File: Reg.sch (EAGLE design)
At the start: 25 parts, among them Q1 NPN, Q2 NPN, Q3 PNP, Q4 NPN, Q5 NPN, Q6 NPN, Q8 PNP

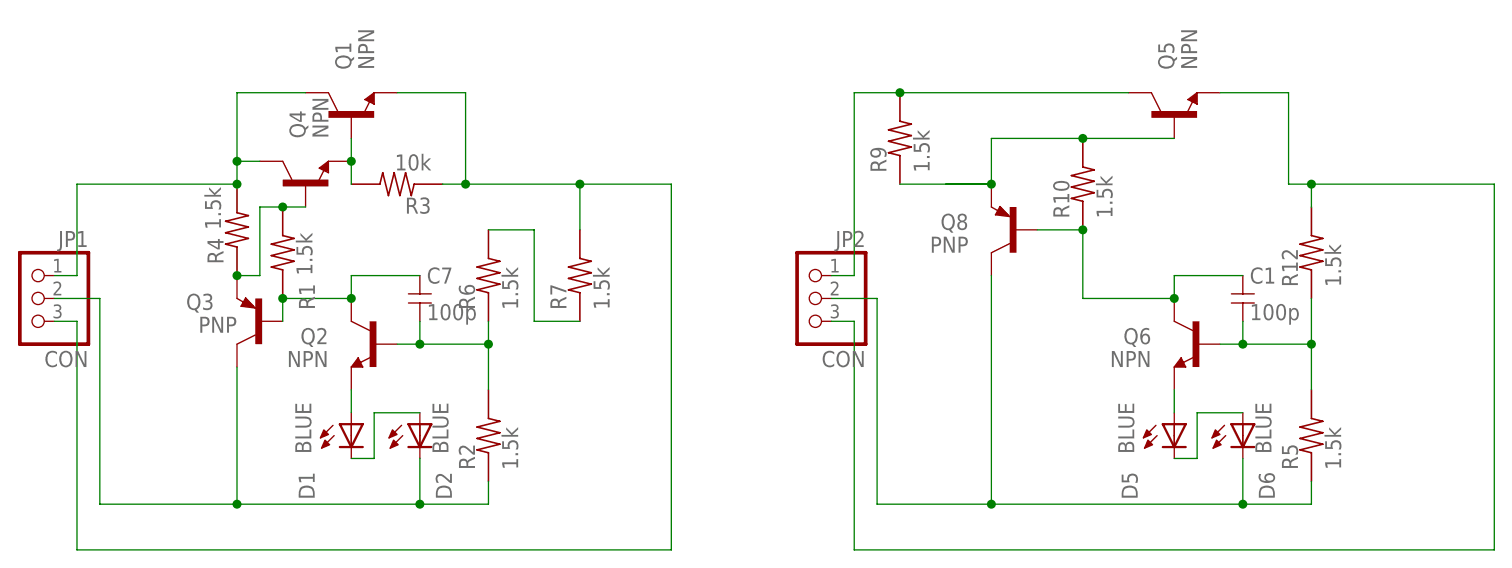
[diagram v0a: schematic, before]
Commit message: シンプルisBest
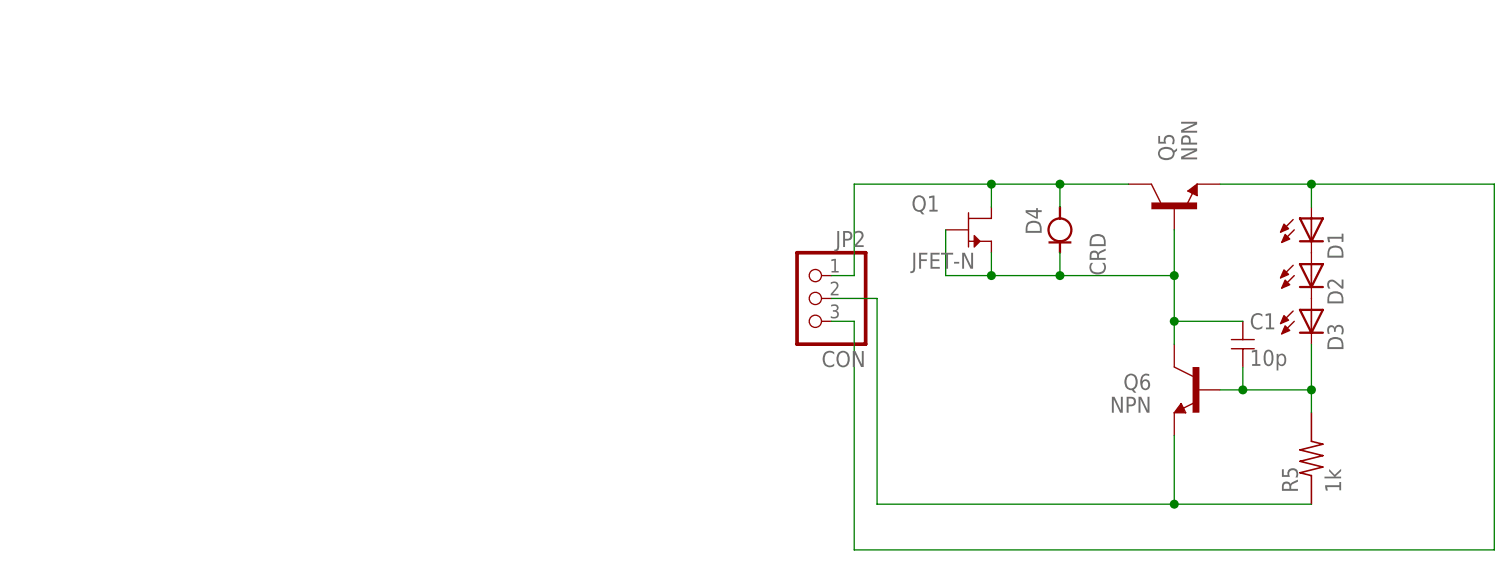
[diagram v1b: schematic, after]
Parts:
- removed C7: 100p, my_rcl:C-1608
- removed D5, D6: BLUE, my_rcl:LED-SMD1608
- removed JP1: CON, pinhead:PINHD-1X3
- removed Q2, Q4: NPN, my_ic:NPN2SC3325
- removed Q3, Q8: PNP, my_ic:PNP2SA1313
- removed R1, R10, R12, R2, R4, R6, R7, R9: 1.5k, my_rcl:R-1608
- removed R3: 10k, my_rcl:R-1608
- added D3: (no value), my_rcl:LED-SMD2012
- added D4: CRD, my_rcl:CRD-SMD
- C1: value 100p -> 10p
- D1, D2: value BLUE -> (none); device my_rcl:LED-SMD1608 -> my_rcl:LED-SMD2012
- JP2: device pinhead:PINHD-1X3 -> my_connector:SW-1X3
- Q1: value NPN -> JFET-N; device my_ic:NPN2SC3422-2 -> my_ic:JFET-N
- Q5: device my_ic:NPN-SOT223 -> my_ic:NPN2SC3422-2
- R5: value 1.5k -> 1k
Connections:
- removed net GND: D2.K, JP1.2, Q3.C, R2.1
- removed net IN: JP1.1, Q1.C, Q4.C, R4.2
- removed net N$1 (its old number): Q3.E, Q4.B, R1.2, R4.1
- removed net N$10: C7.1, Q2.C, Q3.B, R1.1
- removed net N$16: Q5.B, Q8.E, R10.2, R9.1
- removed net N$3: C7.2, Q2.B, R2.2, R6.1
- removed net N$4: D1.A, Q2.E
- removed net N$5: R6.2, R7.1
- removed net N$6: Q1.B, Q4.E, R3.2
- removed net N$8: D5.K, D6.A
- removed net N$9: D5.A, Q6.E
- removed net OUT: JP1.3, Q1.E, R3.1, R7.2
- new net N$2: D2.K, D3.A
- net GND1: now also Q6.E; no longer D6.K, Q8.C
- net IN1: now also D4.A, Q1.D; no longer R9.2
- net N$12: now also D4.K, Q1.G, Q1.S, Q5.B; no longer Q8.B, R10.1
- net N$13: now also D3.K; no longer R12.1
- net OUT1: now also D1.A; no longer R12.2
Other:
- moved on the sheet: C1, D1, D2, Q5, Q6, R5
